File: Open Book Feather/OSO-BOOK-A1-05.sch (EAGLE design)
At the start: 129 parts, among them J1 SJ-43514-SMT, J2 10118193-0001LF, Q1 DMG341, Q2 IRLML0100, SW1 SPDT_SWITCH, U1 AP2112-3.3, U2 MCP73831T-2ACI/OT, U3 ATSAMD51J64-TQFP(10X10), U4 GD25Q16C (or GD25Q32C), U5 74AC165D, U6 GD25Q16C (or GD25Q32C), U7 MAX4468EKAT, X1 JSTPH, X2 2x5 0.05" SWD

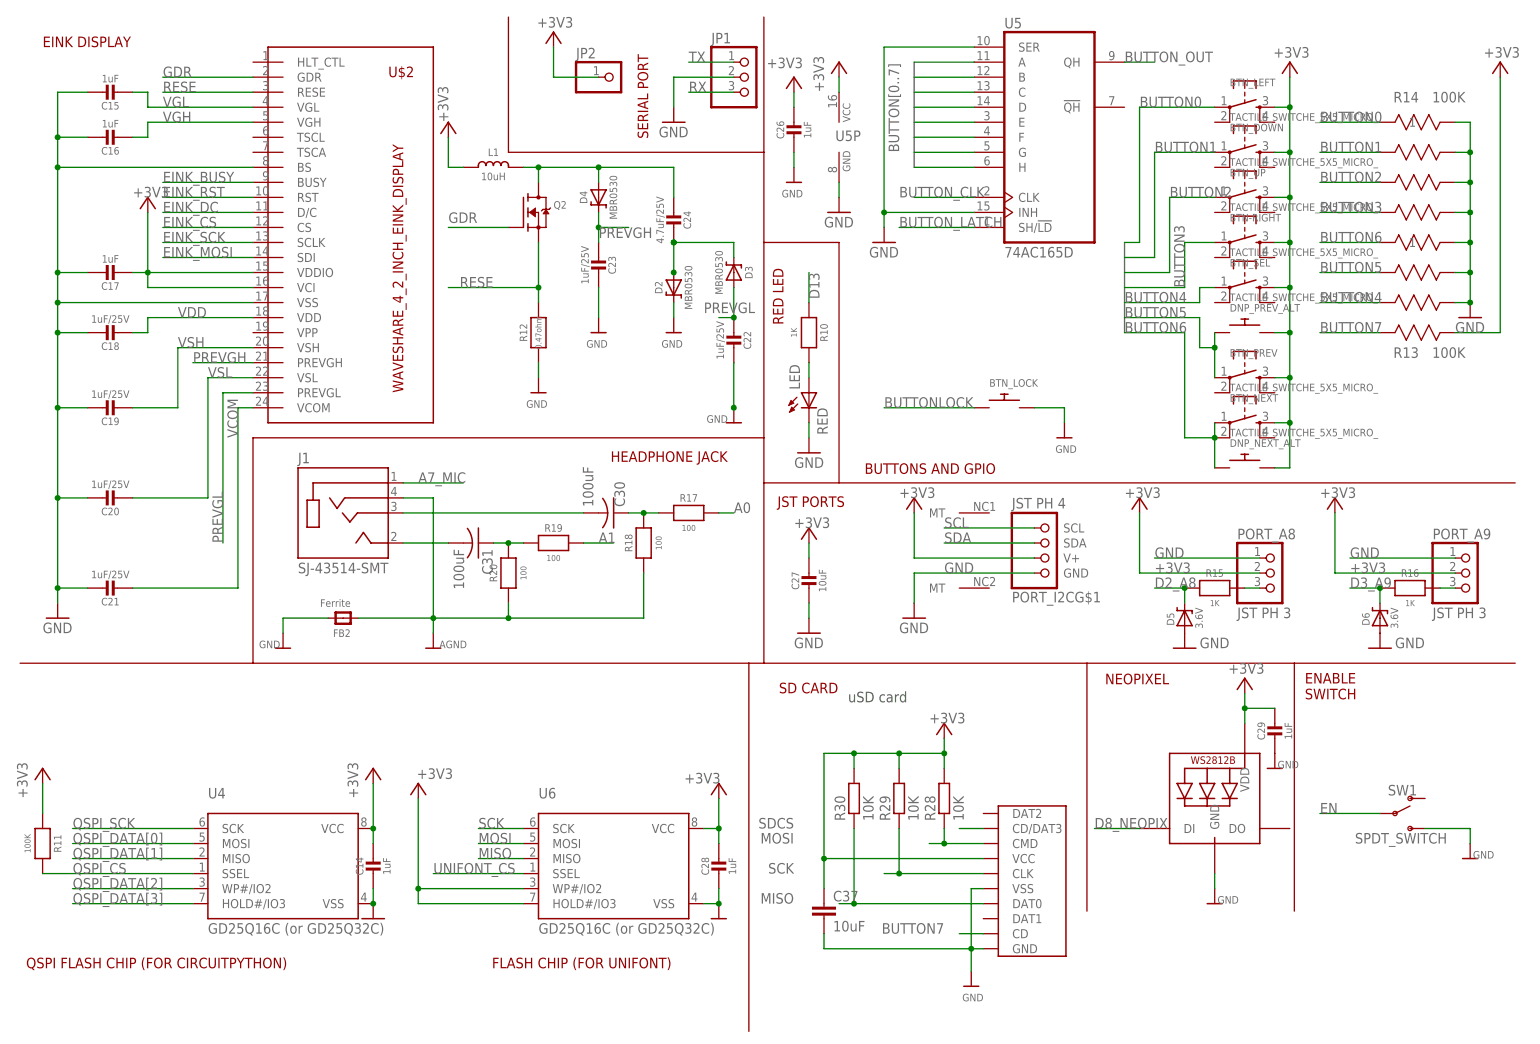
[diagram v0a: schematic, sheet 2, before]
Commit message: Revert "Buttons & SD card change"
This reverts commit 564ec3b5048e0d7899cd32f6cb14d9a07736022d.
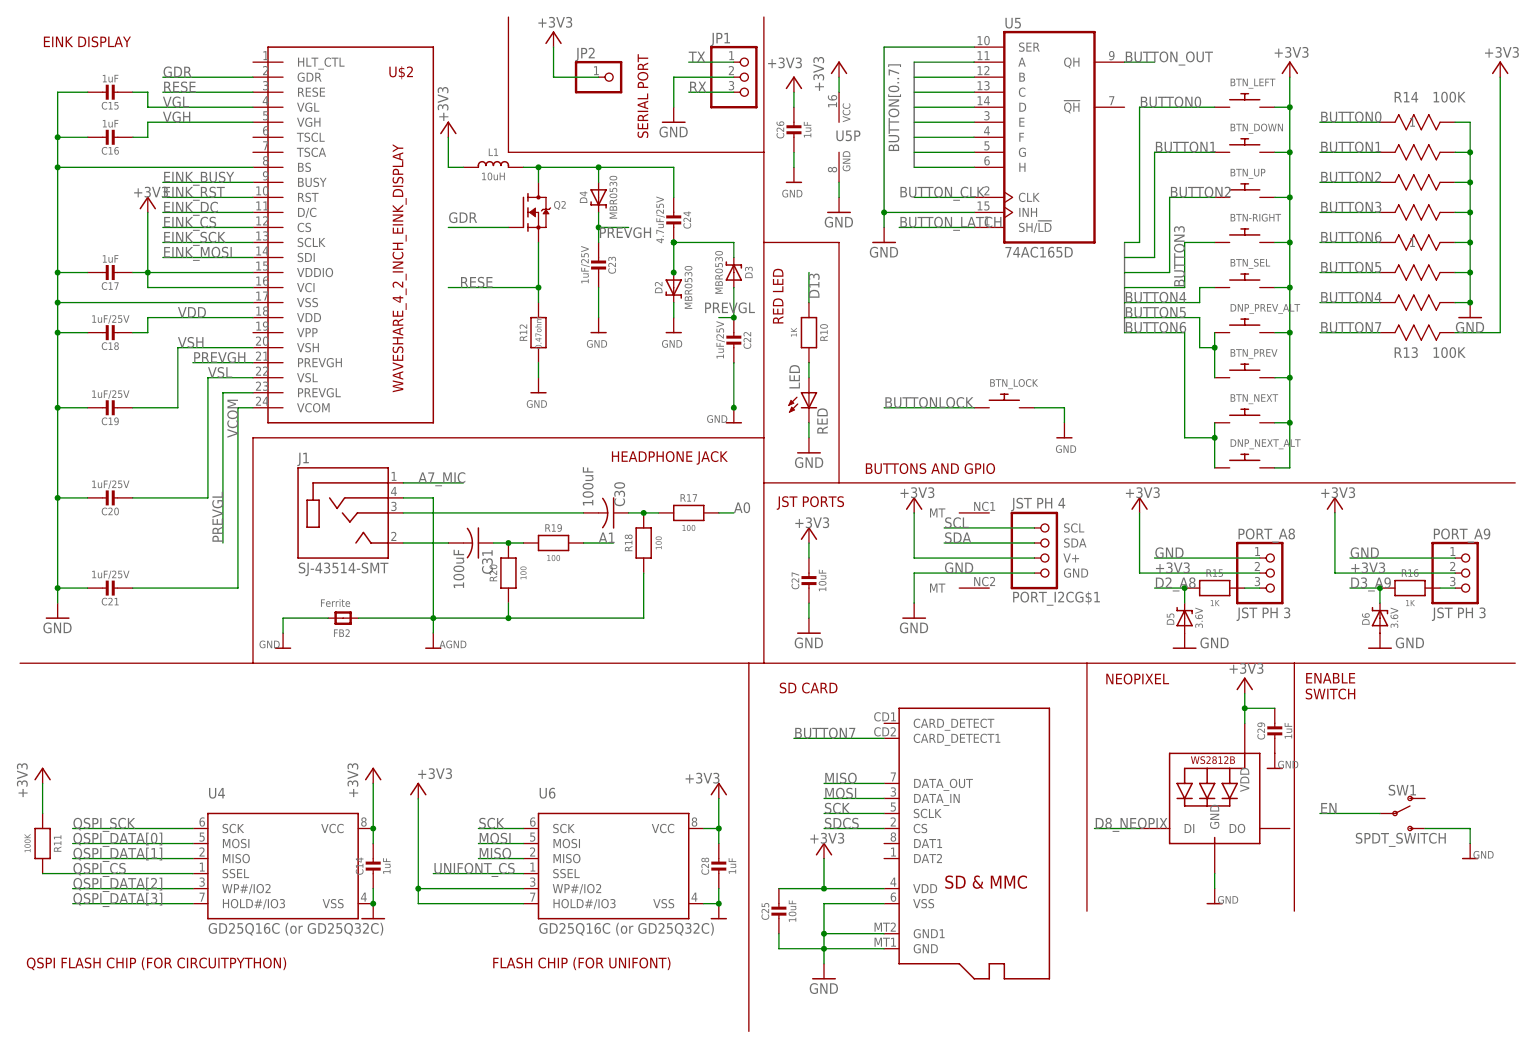
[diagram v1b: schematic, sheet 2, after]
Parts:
- removed C37: 10uF, rcl:C-EUC0805
- removed R28, R29, R30: 10K, rcl:R-EU_R0805
- removed SD_CARD: MICRO_SD_CARD_, dronecz:MICRO_SD_CARD_
- added C25: 10uF, microbuilder:CAP_CERAMIC0805_10MGAP
- added MICROSD: MICROSD, adafruit:MICROSD
- BTN-RIGHT, BTN_DOWN, BTN_LEFT, BTN_NEXT, BTN_PREV, BTN_SEL, BTN_UP: value TACTILE_SWITCHE_5X5_MICRO_ -> (none); device dronecz:TACTILE_SWITCHE_5X5_MICRO_ -> adafruit:SWITCH_PUSHBUTTONEVQ-PE
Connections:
- net +3V3: now also BTN-RIGHT.P$2, BTN_DOWN.P$2, BTN_LEFT.P$2, BTN_NEXT.P$2, BTN_PREV.P$2, BTN_SEL.P$2, BTN_UP.P$2, C25.1, MICROSD.VDD; no longer BTN-RIGHT.3, BTN_DOWN.3, BTN_LEFT.3, BTN_NEXT.3, BTN_PREV.3, BTN_SEL.3, BTN_UP.3, C37.1, R28.2, R29.2, R30.2, SD_CARD.VCC
- net BUTTON0: now also BTN_LEFT.P$1; no longer BTN_LEFT.1
- net BUTTON1: now also BTN_DOWN.P$1; no longer BTN_DOWN.1
- net BUTTON2: now also BTN_UP.P$1; no longer BTN_UP.1
- net BUTTON3: now also BTN-RIGHT.P$1; no longer BTN-RIGHT.1
- net BUTTON4: now also BTN_SEL.P$1; no longer BTN_SEL.1
- net BUTTON5: now also BTN_PREV.P$1; no longer BTN_PREV.1
- net BUTTON6: now also BTN_NEXT.P$1; no longer BTN_NEXT.1, BTN_NEXT.2
- net BUTTON7: now also MICROSD.CARD_DETECT1; no longer SD_CARD.CD
- net GND: now also C25.2, MICROSD.GND, MICROSD.GND1, MICROSD.VSS; no longer C37.2, SD_CARD.GND, SD_CARD.VSS
- net MISO: now also MICROSD.DATA_OUT; no longer R30.1, SD_CARD.DAT0
- net MOSI: now also MICROSD.DATA_IN; no longer R28.1, SD_CARD.CMD
- net SCK: now also MICROSD.SCLK; no longer R29.1, SD_CARD.CLK
- net SDCS: now also MICROSD.CS; no longer SD_CARD.CD/DAT3
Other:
- note removed: "uSD card"
